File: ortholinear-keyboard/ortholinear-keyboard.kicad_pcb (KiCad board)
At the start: 2 copper layers, 214 x 84 mm, 136 parts, among them J1 USB, P1 TC2030-CTX-Tag-Connect, SW1 PG1353, SW10 PG1353, SW11 PG1353, SW12 PG1353, SW13 PG1353, SW14 PG1353, SW15 PG1353, SW16 PG1353, SW17 PG1353, SW18 PG1353, SW19 PG1353, SW2 PG1353, SW20 PG1353, SW21 PG1353, SW22 PG1353, SW23 PG1353, SW24 PG1353, SW25 PG1353, SW26 PG1353, SW27 PG1353, SW28 PG1353, SW29 PG1353, SW3 PG1353, SW30 PG1353, SW31 PG1353, SW32 PG1353, SW33 PG1353, SW34 PG1353, SW35 PG1353, SW36 PG1353, SW37 PG1353, SW38 PG1353, SW39 PG1353, SW4 PG1353, SW40 PG1353, SW41 PG1353, SW42 PG1353, SW43 PG1353, SW44 PG1353, SW45 PG1353, SW46 PG1353, SW47 PG1353, SW48 PG1353, SW49 PG1353, SW5 PG1353, SW50 PG1353, SW51 PG1353, SW52 PG1353, SW53 PG1353, SW54 PG1353, SW55 PG1353, SW56 PG1353, SW57 PG1353, SW58 PG1353, SW59 PG1353, SW6 PG1353, SW60 PG1353, SW7 PG1353, SW8 PG1353, SW9 PG1353, U1 STM32F042K6Ux, U2 XC6206PxxxMR

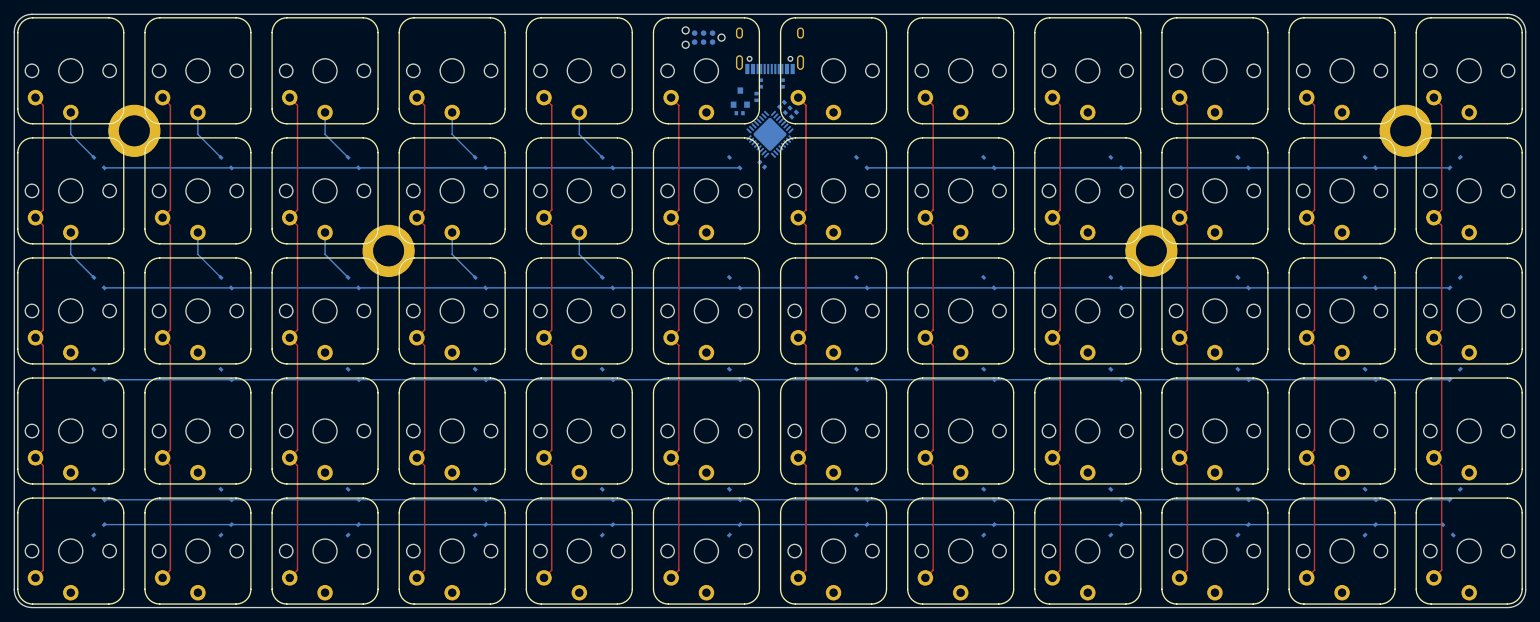
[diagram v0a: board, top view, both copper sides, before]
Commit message: exported production files
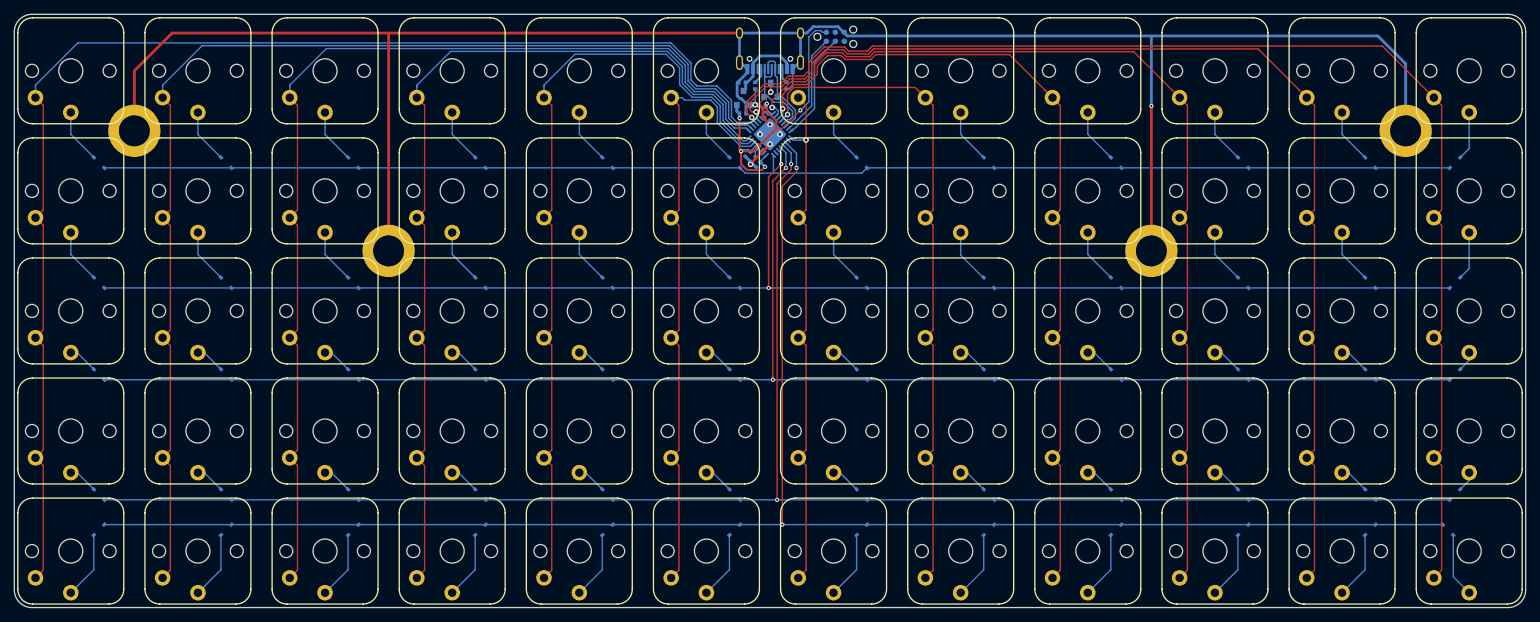
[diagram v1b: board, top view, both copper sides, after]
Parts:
- added D61: SP0502BAHT, Package_TO_SOT_SMD:SOT-23, B.Cu at (157.1, 60.7)
- moved P1 18.7 mm to (166.2, 53.2), turned to 0 degrees
- moved D31 18.0 mm to (170.0, 71.0)
- moved D36 18.0 mm to (188.0, 71.0)
- moved C6 8.71 mm to (155.3, 71.3), turned to 225 degrees
- moved C4 8.52 mm to (153.8, 69.8), turned to 225 degrees
- moved C1 8.50 mm to (154.6, 70.5), turned to 225 degrees
- moved C5 8.40 mm to (155.8, 62.9), turned to 180 degrees
- moved C2 2.90 mm to (153.1, 59.6), turned to 180 degrees
- moved R1 0.85 mm to (154.9, 60.1)
- moved R2 0.58 mm to (159.3, 60.1)
- moved C3 0.45 mm to (153.2, 64.0)
- moved U2 0.45 mm to (153.2, 61.9)
- turned U1 to 45 degrees
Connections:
- U1 pad 10: C5 -> C2
- U1 pad 11: C6 -> C1
- U1 pad 12: C7 -> C12
- U1 pad 13: C8 -> C11
- U1 pad 14: R1 -> Net-(U1-Pad14)
- U1 pad 15: R2 -> Net-(U1-Pad15)
- U1 pad 16: R3 -> Net-(U1-Pad16)
- U1 pad 18: C9 -> C10
- U1 pad 19: C10 -> C9
- U1 pad 20: C11 -> C8
- U1 pad 25: C12 -> C7
- U1 pad 26: R4 -> Net-(U1-Pad26)
- U1 pad 28: Net-(U1-Pad28) -> R4
- U1 pad 29: Net-(U1-Pad29) -> R3
- U1 pad 30: Net-(U1-Pad30) -> R2
- U1 pad 32: Net-(U1-Pad32) -> R1
- U1 pad 6: C1 -> C6
- U1 pad 7: C2 -> C5
- U1 pad 8: C3 -> C4
- U1 pad 9: C4 -> C3
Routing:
- net GND: track 0.00 -> 305.6 mm, vias 0 -> 8
- net C1: track 71.6 -> 185.3 mm
- net C12: track 71.6 -> 180.0 mm, vias 0 -> 1
- net C2: track 71.6 -> 166.7 mm
- net C11: track 71.6 -> 161.1 mm, vias 0 -> 1
- net C3: track 71.6 -> 148.2 mm
- net C10: track 71.6 -> 139.0 mm, vias 0 -> 1
- net C4: track 71.6 -> 130.6 mm
- net R5: track 189.5 -> 245.0 mm, vias 0 -> 2
- net R4: track 190.5 -> 242.0 mm, vias 0 -> 2
- net +3V3: track 0.00 -> 48.4 mm, vias 0 -> 5
- net C9: track 71.6 -> 119.5 mm, vias 0 -> 1
- net C5: track 71.6 -> 112.8 mm
- net R3: track 190.5 -> 224.4 mm, vias 0 -> 2
- net C8: track 71.6 -> 96.4 mm, vias 0 -> 1
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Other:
- board text added: "Ortholinear Keyboard v1.0 @JanHenrikH 2021"
- board text added: "github.com/Jan--Henrik/ortholinear-keyboard-layout"
